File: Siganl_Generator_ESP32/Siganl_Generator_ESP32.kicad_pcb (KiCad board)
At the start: 4 copper layers, 75.7 x 82.4 mm, 20 parts, among them J1 Conn_01x04_Socket, J2 Conn_01x02_Socket, SW1 SW_Push, SW2 SW_Push, SW3 SW_Push, U2 LM393

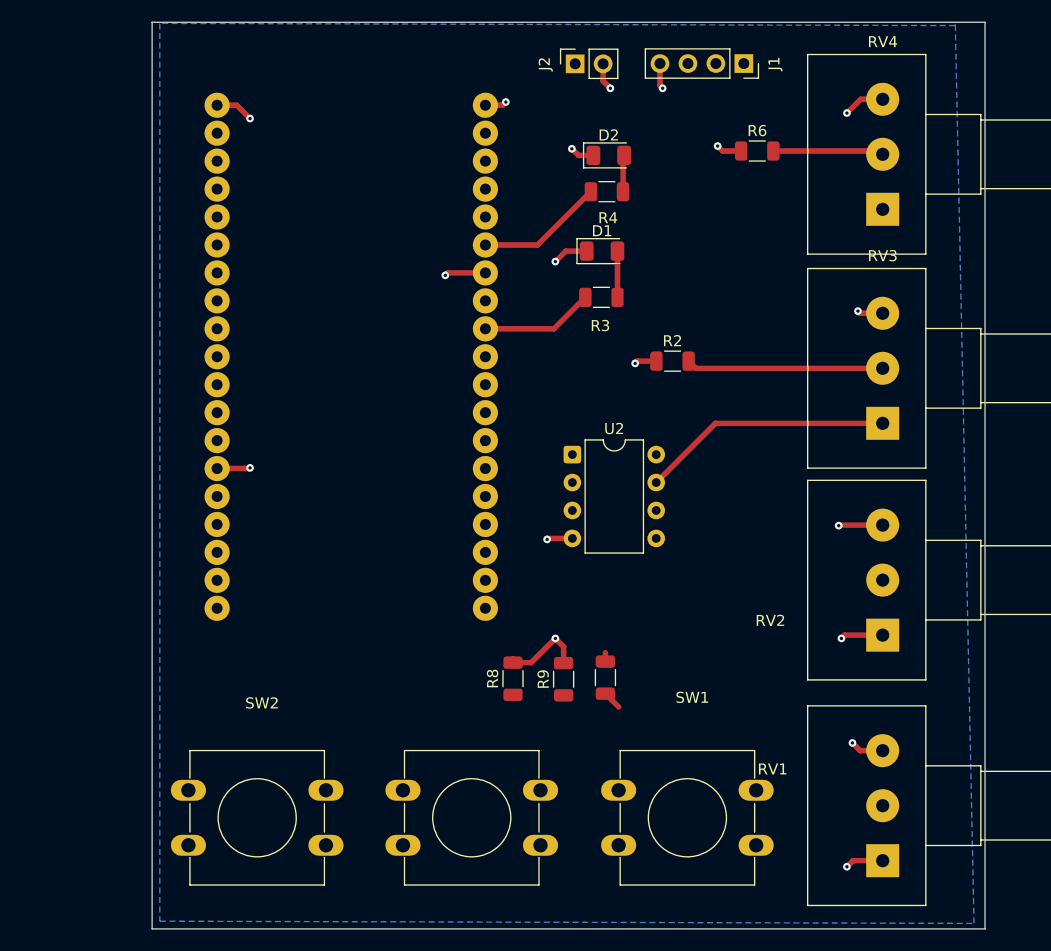
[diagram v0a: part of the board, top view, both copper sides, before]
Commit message: update
design update
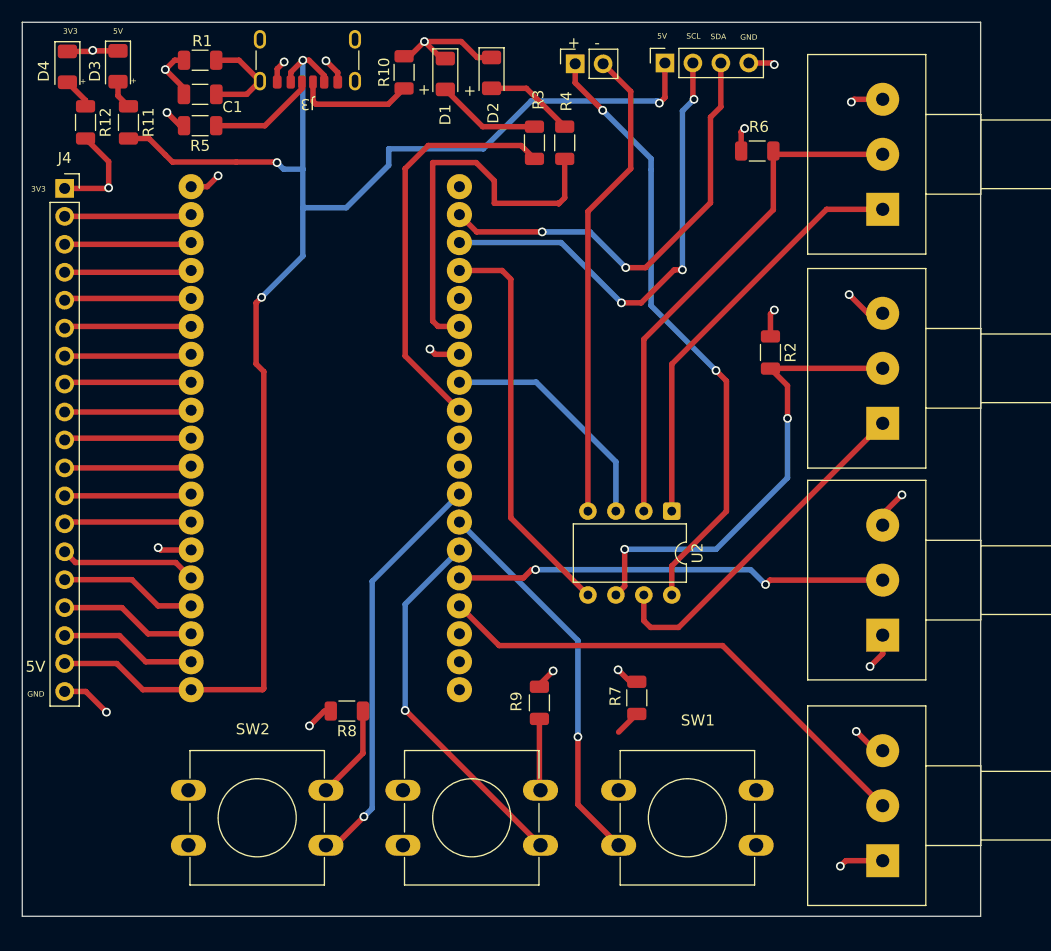
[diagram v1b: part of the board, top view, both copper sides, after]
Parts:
- added C1: 100n, Capacitor_SMD:C_1206_3216Metric, F.Cu at (75.0, 48.0)
- added D3: LED _Red, Diode_SMD:D_1206_3216Metric, F.Cu at (67.5, 45.5)
- added D4: LED_Green, Diode_SMD:D_1206_3216Metric, F.Cu at (62.9, 45.5)
- added J3: USB_C_Receptacle_PowerOnly_6P, Connector_USB:USB_C_Receptacle_GCT_USB4125-xx-x-0190_6P_TopMnt_Horizontal, F.Cu at (84.7, 43.9)
- added J4: Conn_01x19_Socket, Connector_PinSocket_2.54mm:PinSocket_1x19_P2.54mm_Vertical, F.Cu at (62.6, 56.6)
- added R1: 1M, Resistor_SMD:R_1206_3216Metric, F.Cu at (75.0, 45.0)
- added R10: 5K1, Resistor_SMD:R_1206_3216Metric, F.Cu at (93.5, 46.0)
- added R11: 100, Resistor_SMD:R_1206_3216Metric, F.Cu at (68.5, 50.6)
- added R12: 100, Resistor_SMD:R_1206_3216Metric, F.Cu at (64.5, 50.6)
- added R5: 5K1, Resistor_SMD:R_1206_3216Metric, F.Cu at (75.0, 50.9)
- moved D1 21.5 mm to (97.2, 46.2), turned to -90 degrees
- moved R8 15.4 mm to (88.3, 104.1), turned to 180 degrees
- moved R3 15.3 mm to (105.3, 52.5), turned to -90 degrees
- moved D2 13.0 mm to (101.5, 46.1), turned to -90 degrees
- moved U2 10.4 mm to (117.8, 85.9), turned to -90 degrees
- moved R2 8.93 mm to (126.8, 71.5), turned to -90 degrees
- moved U1 7.77 mm to (93.5, 66.6)
- moved J1 7.17 mm to (117.2, 45.2), turned to 90 degrees
- moved R4 5.88 mm to (108.1, 52.5), turned to -90 degrees
- moved R7 3.39 mm to (114.7, 102.9)
- moved R9 3.07 mm to (105.8, 103.3)
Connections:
- J1 pad 1: VCC -> 5 V
- J2 pad 1: VCC -> 12 V
- J2 pad 2: GND -> -12 V
- U1 pad 10: unconnected-(U1-G26-Pad10) -> Net-(J4-Pin_10)
- U1 pad 11: unconnected-(U1-G27-Pad11) -> Net-(J4-Pin_11)
- U1 pad 12: Signal 2 -> Net-(J4-Pin_12)
- U1 pad 13: unconnected-(U1-G12-Pad13) -> Net-(J4-Pin_13)
- U1 pad 15: unconnected-(U1-G13-Pad15) -> Net-(J4-Pin_14)
- U1 pad 16: unconnected-(U1-SD2-Pad16) -> Net-(J4-Pin_15)
- U1 pad 17: unconnected-(U1-SD3-Pad17) -> Net-(J4-Pin_16)
- U1 pad 18: Signal 1 -> Net-(J4-Pin_17)
- U1 pad 19: VCC -> 5 V
- U1 pad 2: unconnected-(U1-EN-Pad2) -> Net-(J4-Pin_2)
- U1 pad 23: unconnected-(U1-TDX-Pad23) -> Signal 1
- U1 pad 27: unconnected-(U1-G19-Pad27) -> Signal 2
- U1 pad 3: unconnected-(U1-SP-Pad3) -> Net-(J4-Pin_3)
- U1 pad 4: unconnected-(U1-SN-Pad4) -> Net-(J4-Pin_4)
- U1 pad 5: unconnected-(U1-G34-Pad5) -> Net-(J4-Pin_5)
- U1 pad 6: unconnected-(U1-G35-Pad6) -> Net-(J4-Pin_6)
- U1 pad 7: unconnected-(U1-G32-Pad7) -> Net-(J4-Pin_7)
- U1 pad 8: unconnected-(U1-G33-Pad8) -> Net-(J4-Pin_8)
- U1 pad 9: unconnected-(U1-G25-Pad9) -> Net-(J4-Pin_9)
- U2 pad 4: GND -> -12 V
- U2 pad 8: VCC -> 12 V
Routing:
- net 5 V: track 0.00 -> 142.1 mm, vias 0 -> 4
- net 12 V: track 0.00 -> 56.0 mm, vias 0 -> 2
- net G35 DutyCycle: track 0.00 -> 46.0 mm
- net -12 V: track 0.00 -> 43.3 mm
- net OLED_SCL: track 0.00 -> 43.1 mm, vias 0 -> 3
- net OLED_SDA: track 0.00 -> 40.3 mm, vias 0 -> 2
- net G34 Frquenz: track 0.00 -> 39.5 mm, vias 0 -> 2
- net Net-(RV4-Pad1): track 0.00 -> 38.4 mm
- net Net-(U2A--): track 10.1 -> 47.7 mm
- net Buttom 2: track 0.00 -> 37.4 mm, vias 0 -> 1
- net Signal 1: track 0.00 -> 36.6 mm
- net Buttom 1_Siganl_Switch: track 0.00 -> 35.4 mm
- net Buttom 3: track 0.00 -> 34.0 mm, vias 0 -> 1
- net Led_Red: track 10.3 -> 37.1 mm
- net Net-(U2B--): track 17.9 -> 42.8 mm, vias 0 -> 2
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- added copper zone on In2.Cu, net 3V3
- added copper zone on In1.Cu, net GND
- removed copper zone on B.Cu, net GND
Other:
- board size 75.7 x 82.4 mm -> 87.1 x 81.2 mm
- board text added: "+"
- board text added: "-"
- board text added: "3V3"
- board text added: "5V"
- board text added: "GND"
- board text added: "R7"
- board text added: "SCL"
- board text added: "SDA"
- board text added: "Siganl Gererater v.1 designed by Amjad Trablsi"

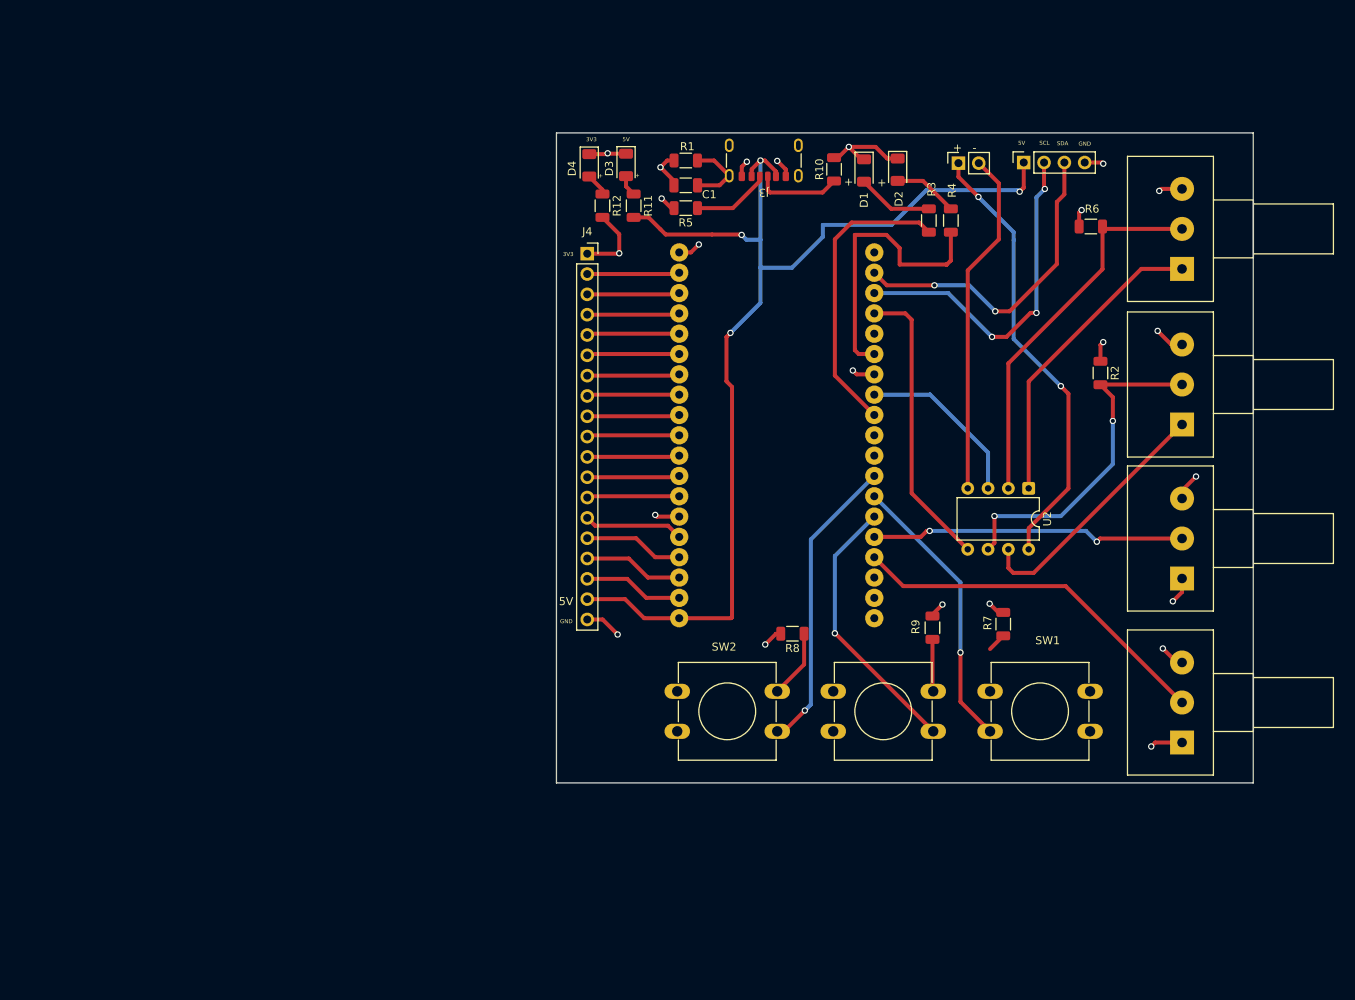
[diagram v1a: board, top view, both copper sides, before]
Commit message: klein update
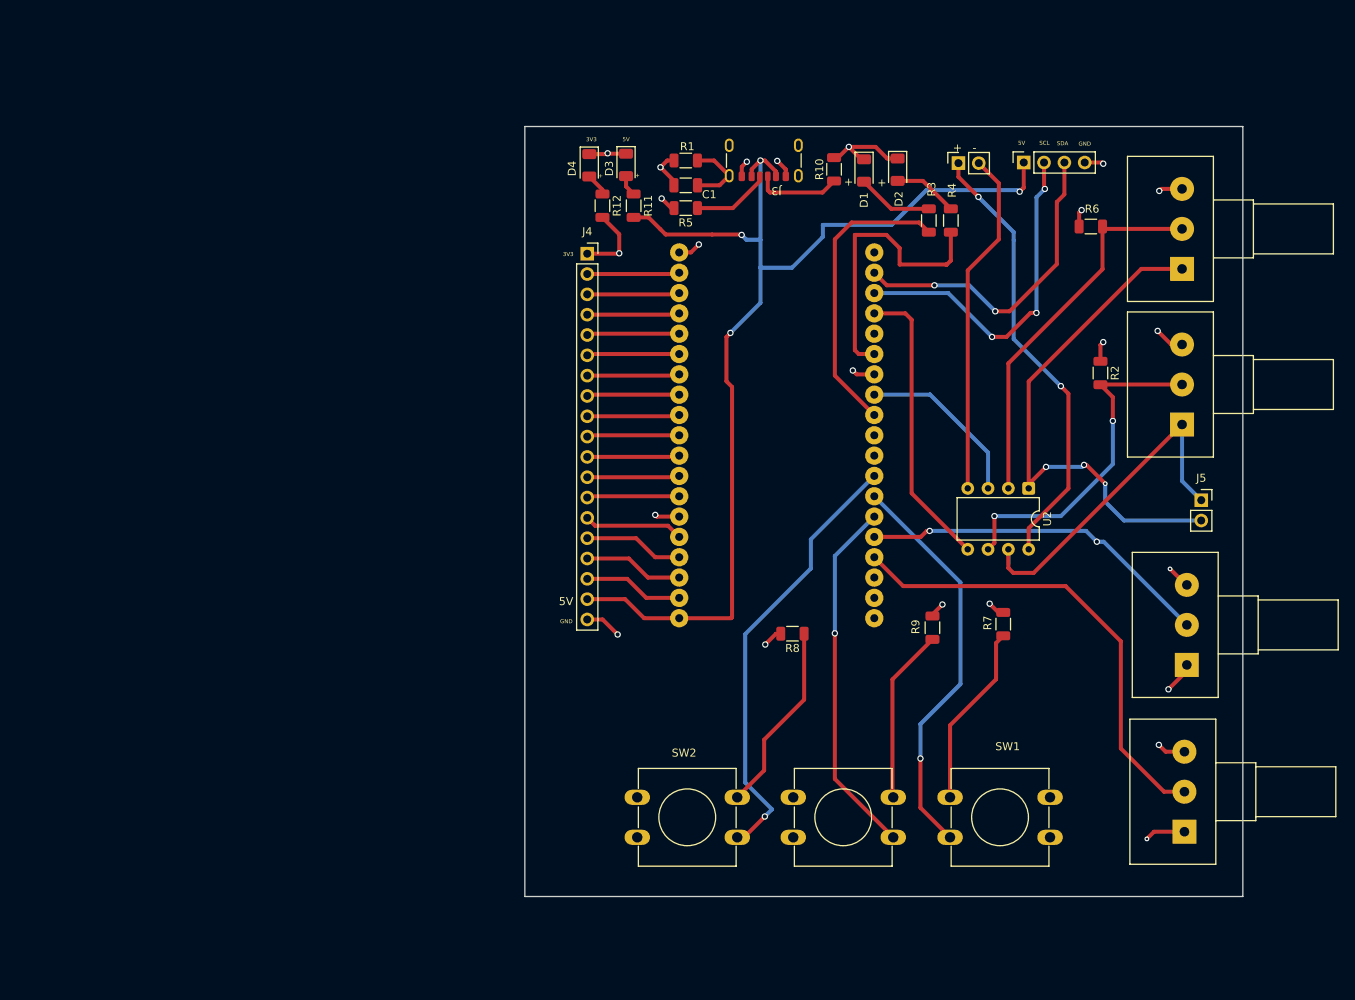
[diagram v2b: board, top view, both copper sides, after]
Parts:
- added J5: Conn_01x02_Socket, Connector_PinSocket_2.54mm:PinSocket_1x02_P2.54mm_Vertical, F.Cu at (139.4, 87.4)
- moved SW1 14.2 mm to (108.0, 124.5)
- moved SW2 14.2 mm to (68.9, 124.5)
- moved SW3 14.2 mm to (88.4, 124.5)
- moved RV1 11.2 mm to (137.3, 128.8)
- moved RV2 10.8 mm to (137.6, 108.0)
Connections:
- net Net-(RV3-Pad1) renamed Signal 1 Output
- net Net-(RV4-Pad1) renamed Siganl 2 Output
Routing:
- net Siganl 2 Output: track 38.4 -> 65.6 mm, vias 0 -> 3
- net Net-(R7-Pad1): track 2.33 -> 22.9 mm
- net Buttom 2: track 37.4 -> 55.5 mm
- net Buttom 1_Siganl_Switch: track 35.4 -> 50.7 mm
- net Net-(R9-Pad1): track 6.39 -> 21.7 mm
- net Net-(R8-Pad1): track 8.59 -> 23.9 mm
- net G35 DutyCycle: track 46.0 -> 58.8 mm
- net Signal 1 Output: track 32.0 -> 44.4 mm
- net Buttom 3: track 34.0 -> 45.2 mm
- net G34 Frquenz: track 39.5 -> 44.2 mm
- net 3V3: track 19.6 -> 21.3 mm
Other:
- board size 87.1 x 81.2 mm -> 89.8 x 96.2 mm

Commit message: update
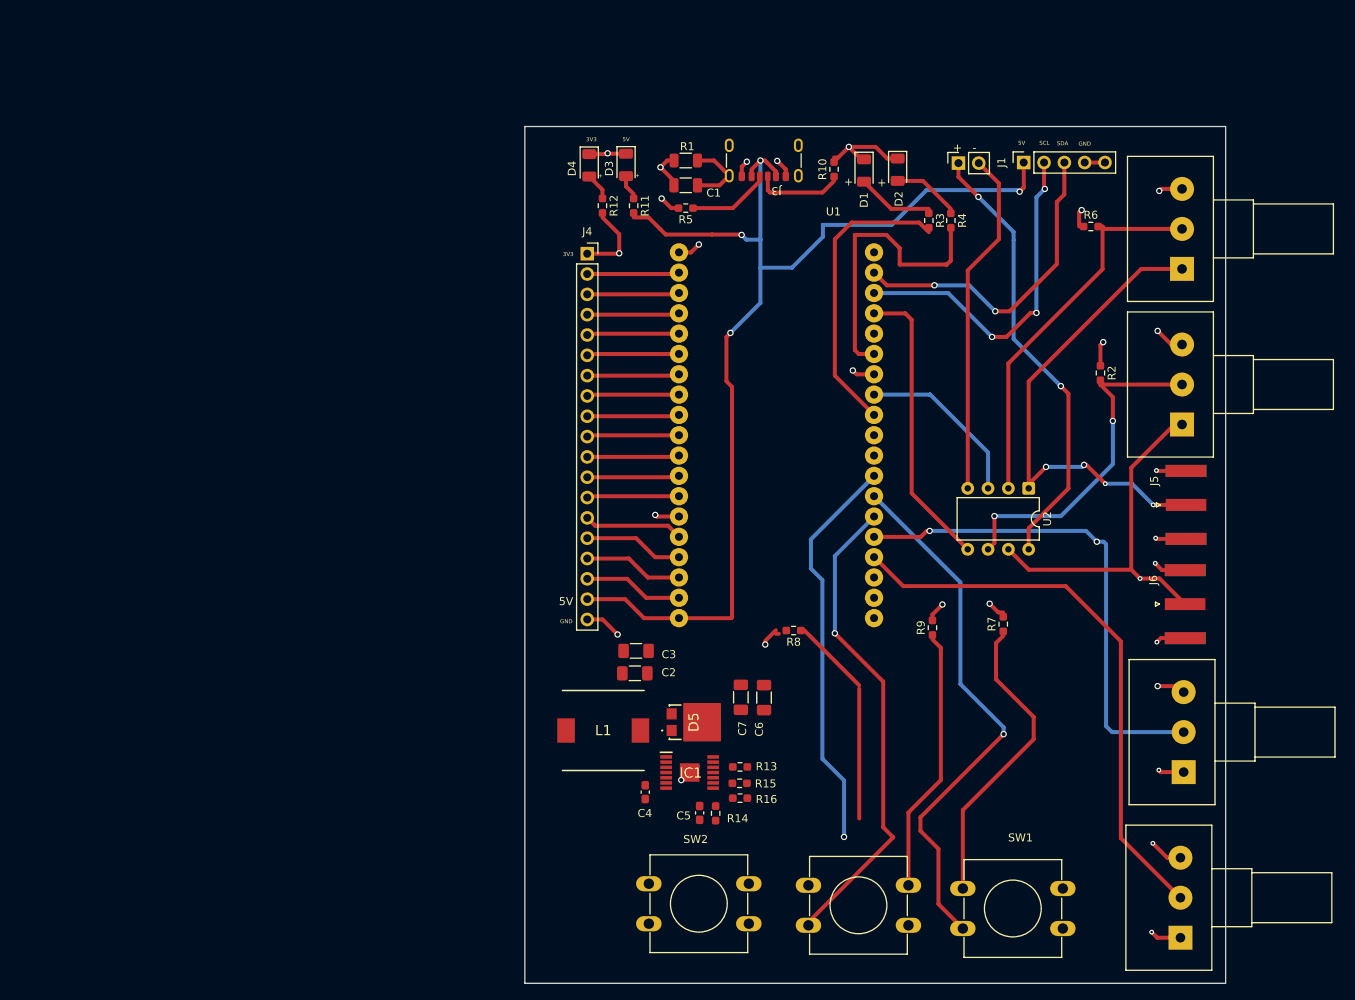
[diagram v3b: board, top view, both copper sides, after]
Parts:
- added C2: 4u7, Capacitor_SMD:C_1206_3216Metric_Pad1.33x1.80mm_HandSolder, F.Cu at (68.6, 109.0)
- added C3: 4u7, Capacitor_SMD:C_1206_3216Metric_Pad1.33x1.80mm_HandSolder, F.Cu at (68.8, 106.2)
- added C4: 100n, Capacitor_SMD:C_0603_1608Metric_Pad1.08x0.95mm_HandSolder, F.Cu at (69.9, 123.9)
- added C5: 1n, Capacitor_SMD:C_0603_1608Metric_Pad1.08x0.95mm_HandSolder, F.Cu at (76.7, 126.5)
- added C6: 4u7, Capacitor_SMD:C_1206_3216Metric_Pad1.33x1.80mm_HandSolder, F.Cu at (84.8, 112.1)
- added C7: 4u7, Capacitor_SMD:C_1206_3216Metric_Pad1.33x1.80mm_HandSolder, F.Cu at (81.8, 112.0)
- added D5: SS3P6L-E3_86A, Amjad_lib:SS3P6LE386A, F.Cu at (76.0, 115.2)
- added IC1: TPS61175QPWPRQ1, Amjad_lib:SOP65P640X120-15N, F.Cu at (75.5, 121.5)
- added J6: Conn_Coaxial, Connector_Coaxial:SMA_Amphenol_132289_EdgeMount, F.Cu at (137.4, 100.4)
- added L1: CDRH105RNP-220NC, Amjad_lib:INDPM102100X510N_Spule, F.Cu at (64.7, 116.2)
- added R13: 51k, Resistor_SMD:R_0603_1608Metric_Pad0.98x0.95mm_HandSolder, F.Cu at (81.8, 120.8)
- added R14: 1k, Resistor_SMD:R_0603_1608Metric_Pad0.98x0.95mm_HandSolder, F.Cu at (78.7, 126.5)
- added R15: 200K, Resistor_SMD:R_0603_1608Metric_Pad0.98x0.95mm_HandSolder, F.Cu at (81.7, 122.8)
- added R16: 10K, Resistor_SMD:R_0603_1608Metric_Pad0.98x0.95mm_HandSolder, F.Cu at (81.8, 124.7)
- J1: value Conn_01x04_Socket -> Conn_01x05_Socket; footprint Connector_PinSocket_2.54mm:PinSocket_1x04_P2.54mm_Vertical -> Connector_PinSocket_2.54mm:PinSocket_1x05_P2.54mm_Vertical
- J5: value Conn_01x02_Socket -> Conn_Coaxial; footprint Connector_PinSocket_2.54mm:PinSocket_1x02_P2.54mm_Vertical -> Connector_Coaxial:SMA_Amphenol_132289_EdgeMount
- R10, R11, R12, R2, R3, R4, R5, R6, R7, R8, R9: footprint Resistor_SMD:R_1206_3216Metric -> Resistor_SMD:R_0603_1608Metric_Pad0.98x0.95mm_HandSolder
- moved RV2 13.4 mm to (137.2, 121.4)
- moved RV1 13.3 mm to (136.8, 142.1)
- moved SW1 11.5 mm to (109.6, 135.9)
- moved SW3 11.2 mm to (90.3, 135.6)
- moved SW2 10.9 mm to (70.3, 135.3)
- moved J5 1.99 mm to (137.5, 88.0)
- moved R8 0.42 mm to (88.4, 103.7)
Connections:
- J1 pad 4: GND -> CS
- J5 pad 1: Signal 1 Output -> Siganl 2 Output
- J5 pad 2: Siganl 2 Output -> GND
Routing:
- net GND: track 65.0 -> 84.5 mm, vias 19 -> 24
- net G34 Frquenz: track 44.2 -> 62.7 mm
- net Buttom 1_Siganl_Switch: track 50.7 -> 67.2 mm
- net Buttom 3: track 45.2 -> 60.6 mm
- net Net-(R7-Pad1): track 22.9 -> 37.6 mm
- net G35 DutyCycle: track 58.8 -> 70.3 mm
- net Net-(R9-Pad1): track 21.7 -> 32.8 mm
- net Buttom 2: track 55.5 -> 50.1 mm
- net Siganl 2 Output: track 65.6 -> 61.6 mm, vias 3 -> 4
- net Net-(R8-Pad1): track 23.9 -> 26.0 mm
- net 3V3: track 21.3 -> 19.3 mm
- net Signal 1 Output: track 44.4 -> 46.3 mm, vias 0 -> 1
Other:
- board size 89.8 x 96.2 mm -> 87.6 x 107.1 mm
- board text removed: "R7"
